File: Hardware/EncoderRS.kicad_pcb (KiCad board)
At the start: 2 copper layers, 38 x 38 mm, 31 parts, among them J1 Conn_01x04, J2 Conn_01x04, U1 STM8S003F3P, U2 SP3485EN, U3 MT6816CT-ACD, U4 HT75R33-1A, Y1 X1E0000210119

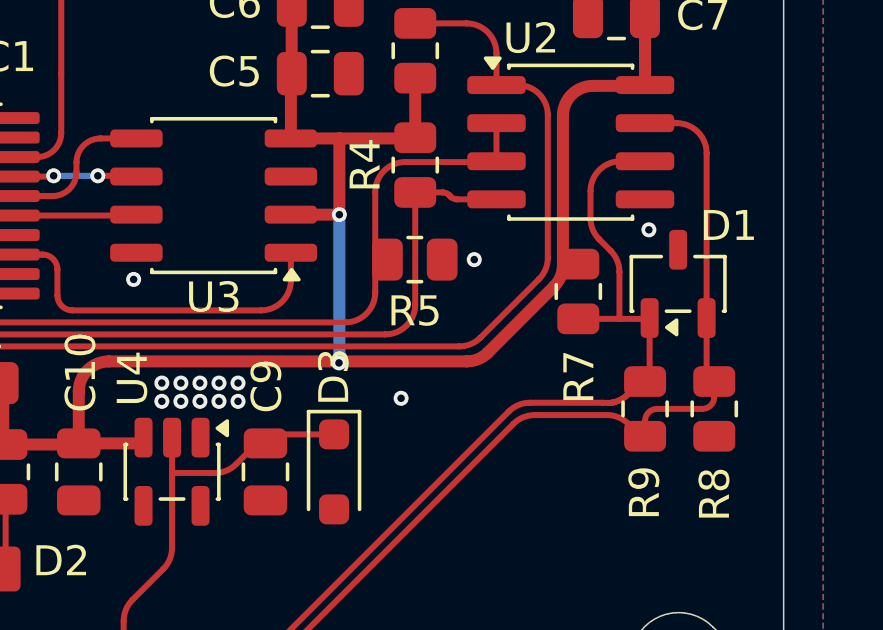
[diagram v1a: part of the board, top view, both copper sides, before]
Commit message: Updated libs
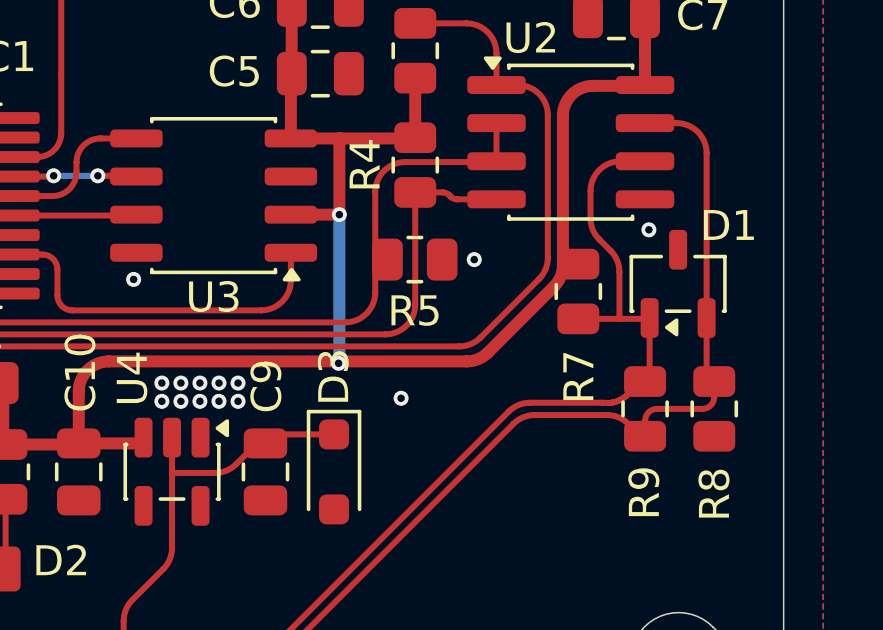
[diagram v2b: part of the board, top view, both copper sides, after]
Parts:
- D2: footprint LED_SMD:LED_1206_3216Metric_ReverseMount_Hole1.8x2.4mm -> encoders_lib:LED_1206_3216Metric_ReverseMount_Hole2.1mm
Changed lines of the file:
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@@
 		)
 	)
-	(footprint "LED_SMD:LED_1206_3216Metric_ReverseMount_Hole1.8x2.4mm"
+	(footprint "encoders_lib:LED_1206_3216Metric_ReverseMount_Hole2.1mm"
 		(layer "F.Cu")
 		(at 32.7898 53.321)
@@
 	)
 	(segment
+		(start 55.266226 37.1901)
+		(end 55.7532 37.1901)
+		(width 0.4)
+		(layer "F.Cu")
+		(net 2)
+	)
+	(segment
+		(start 54.016889 37.2174)
+		(end 55.238926 37.2174)
+		(width 0.4)
+		(layer "F.Cu")
+		(net 2)
+	)
+	(segment
 		(start 43.95 38.97)
 		(end 43.95 36.837)
@@
 	)
 	(segment
+		(start 55.238926 37.2174)
+		(end 55.266226 37.1901)
+		(width 0.4)
+		(layer "F.Cu")
+		(net 2)
+	)
+	(segment
 		(start 43.981 34.52)
 		(end 43.976 34.525)
@@
 	)
 	(segment
-		(start 45.6025 46.402)
-		(end 49.810186 46.402)
+		(start 34.4662 49.1725)
+		(end 36.8417 49.1725)
 		(width 0.4)
 		(layer "F.Cu")
@@
 	)
 	(segment
-		(start 53.016889 43.195297)
-		(end 53.016889 38.2174)
+		(start 45.539637 46.464863)
+		(end 45.539637 46.439137)
 		(width 0.4)
 		(layer "F.Cu")
@@
 	)
 	(segment
-		(start 34.4662 49.1725)
-		(end 36.8417 49.1725)
+		(start 45.6025 46.402)
+		(end 49.810186 46.402)
+		(width 0.4)
+		(layer "F.Cu")
+		(net 2)
+	)
+	(segment
+		(start 45.539637 46.439137)
+		(end 45.5025 46.402)
 		(width 0.4)
 		(layer "F.Cu")
@@
 	)
 	(segment
-		(start 45.5525 46.452)
-		(end 45.6025 46.402)
-		(width 0.4)
-		(layer "F.Cu")
-		(net 2)
-	)
-	(segment
-		(start 55.238926 37.2174)
-		(end 55.266226 37.1901)
+		(start 36.8792 47.402)
+		(end 36.8792 49.135)
 		(width 0.4)
 		(layer "F.Cu")
@@
 	)
 	(segment
-		(start 36.8792 47.402)
-		(end 36.8792 49.135)
+		(start 53.016889 43.195297)
+		(end 53.016889 38.2174)
 		(width 0.4)
 		(layer "F.Cu")
@@
 	)
 	(segment
-		(start 43.683107 27.954707)
-		(end 40.0034 24.275)
+		(start 50.517293 46.109107)
+		(end 52.723996 43.902404)
 		(width 0.4)
 		(layer "F.Cu")
@@
 	)
 	(segment
-		(start 32.523893 48.737093)
-		(end 32.666407 48.879607)
+		(start 43.683107 27.954707)
+		(end 40.0034 24.275)
 		(width 0.4)
 		(layer "F.Cu")
@@
 	)
 	(segment
-		(start 45.5525 46.452)
-		(end 45.5025 46.402)
+		(start 32.523893 48.737093)
+		(end 32.666407 48.879607)
 		(width 0.4)
 		(layer "F.Cu")
@@
 	)
 	(segment
-		(start 55.266226 37.1901)
-		(end 55.7532 37.1901)
-		(width 0.4)
-		(layer "F.Cu")
-		(net 2)
-	)
-	(segment
 		(start 43.976 34.271)
 		(end 43.976 28.661814)
@@
 	)
 	(segment
-		(start 54.016889 37.2174)
-		(end 55.238926 37.2174)
-		(width 0.4)
-		(layer "F.Cu")
-		(net 2)
-	)
-	(segment
 		(start 33.373514 49.1725)
 		(end 34.4662 49.1725)
@@
 	)
 	(segment
+		(start 45.539637 46.464863)
+		(end 45.6025 46.402)
+		(width 0.4)
+		(layer "F.Cu")
+		(net 2)
+	)
+	(segment
 		(start 45.566 41.51)
 		(end 45.566 38.97)
@@
 	)
 	(segment
-		(start 50.517293 46.109107)
-		(end 52.723996 43.902404)
-		(width 0.4)
-		(layer "F.Cu")
-		(net 2)
-	)
-	(segment
 		(start 45.566 38.97)
 		(end 43.95 38.97)
@@
 	)
 	(via
-		(at 45.5525 46.452)
+		(at 45.539637 46.464863)
 		(size 0.5)
 		(drill 0.25)
@@
 	)
 	(arc
+		(start 37.8792 46.402)
+		(mid 37.172093 46.694893)
+		(end 36.8792 47.402)
+		(width 0.4)
+		(layer "F.Cu")
+		(net 2)
+	)
+	(arc
 		(start 32.666407 48.879607)
 		(mid 32.99083 49.09638)
@@
 	)
 	(arc
-		(start 53.016889 43.195297)
-		(mid 52.940769 43.57798)
-		(end 52.723996 43.902404)
+		(start 49.810186 46.402)
+		(mid 50.192869 46.32588)
+		(end 50.517293 46.109107)
 		(width 0.4)
 		(layer "F.Cu")
@@
 	)
 	(arc
-		(start 49.810186 46.402)
-		(mid 50.192869 46.32588)
-		(end 50.517293 46.109107)
+		(start 53.016889 38.2174)
+		(mid 53.309782 37.510293)
+		(end 54.016889 37.2174)
 		(width 0.4)
 		(layer "F.Cu")
@@
 	)
 	(arc
-		(start 37.8792 46.402)
-		(mid 37.172093 46.694893)
-		(end 36.8792 47.402)
+		(start 52.723996 43.902404)
+		(mid 52.940769 43.57798)
+		(end 53.016889 43.195297)
 		(width 0.4)
 		(layer "F.Cu")
 		(net 2)
 	)
-	(arc
-		(start 53.016889 38.2174)
-		(mid 53.309782 37.510293)
-		(end 54.016889 37.2174)
-		(width 0.4)
-		(layer "F.Cu")
+	(segment
+		(start 45.539637 46.464863)
+		(end 45.5525 46.452)
+		(width 0.2)
+		(layer "B.Cu")
 		(net 2)
 	)
@@
 	)
 	(segment
-		(start 45.5525 46.402)
-		(end 45.566 46.3885)
+		(start 45.5525 46.452)
+		(end 45.5525 46.402)
 		(width 0.2)
 		(layer "B.Cu")
@@
 	)
 	(segment
-		(start 45.5525 46.452)
-		(end 45.5525 46.402)
+		(start 45.5525 46.402)
+		(end 45.566 46.3885)
 		(width 0.2)
 		(layer "B.Cu")
@@
 	)
 	(zone
-		(net 21)
-		(net_name "/NRST")
+		(net 2)
+		(net_name "+3V3")
 		(layer "F.Cu")
 		(name "$teardrop_padvia$")
 		(hatch none 0.1)
-		(priority 30006)
+		(priority 30000)
 		(attr
 			(teardrop
@@
 		(polygon
 			(pts
-				(xy 31.253239 39.6542) (xy 31.253239 39.4542) (xy 30.810627 39.512204) (xy 30.8584 39.7574) (xy 31.067267 39.896293)
+				(xy 45.050277 46.202) (xy 45.050277 46.602) (xy 45.490864 46.710059) (xy 45.540637 46.464863) (xy 45.58841 46.219667)
 			)
 		)
 	)
 	(zone
-		(net 2)
-		(net_name "+3V3")
+		(net 21)
+		(net_name "/NRST")
 		(layer "F.Cu")
 		(name "$teardrop_padvia$")
 		(hatch none 0.1)
-		(priority 30000)
+		(priority 30006)
 		(attr
 			(teardrop
@@
 		(polygon
 			(pts
-				(xy 45.057812 46.202) (xy 45.057812 46.602) (xy 45.503727 46.697196) (xy 45.5535 46.452) (xy 45.601273 46.206804)
+				(xy 31.253239 39.6542) (xy 31.253239 39.4542) (xy 30.810627 39.512204) (xy 30.8584 39.7574) (xy 31.067267 39.896293)
 			)
 		)
@@
 	)
 	(zone
-		(net 21)
-		(net_name "/NRST")
+		(net 2)
+		(net_name "+3V3")
 		(layer "F.Cu")
 		(name "$teardrop_padvia$")
 		(hatch none 0.1)
-		(priority 30004)
+		(priority 30001)
 		(attr
 			(teardrop
@@
 		(polygon
 			(pts
-				(xy 30.9594 37.027004) (xy 30.7594 37.027004) (xy 30.614204 37.473427) (xy 30.8594 37.5232) (xy 31.104596 37.473427)
+				(xy 46.028997 46.602) (xy 46.028997 46.202) (xy 45.490864 46.219667) (xy 45.538637 46.464863) (xy 45.58841 46.710059)
 			)
 		)
 	)
 	(zone
-		(net 2)
-		(net_name "+3V3")
+		(net 21)
+		(net_name "/NRST")
 		(layer "F.Cu")
 		(name "$teardrop_padvia$")
 		(hatch none 0.1)
-		(priority 30001)
+		(priority 30004)
 		(attr
 			(teardrop
@@
 		(polygon
 			(pts
-				(xy 46.047188 46.602) (xy 46.047188 46.202) (xy 45.503727 46.206804) (xy 45.5515 46.452) (xy 45.601273 46.697196)
+				(xy 30.9594 37.027004) (xy 30.7594 37.027004) (xy 30.614204 37.473427) (xy 30.8594 37.5232) (xy 31.104596 37.473427)
 			)
 		)
@@
 		(polygon
 			(pts
-				(xy 45.766 45.956804) (xy 45.366 45.956804) (xy 45.307304 46.403227) (xy 45.5525 46.453) (xy 45.797696 46.403227)
+				(xy 45.766 45.969667) (xy 45.366 45.969667) (xy 45.294441 46.41609) (xy 45.539637 46.465863) (xy 45.784833 46.41609)
 			)
 		)
